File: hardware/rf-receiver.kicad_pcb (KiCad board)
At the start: 4 copper layers, 90.8 x 50 mm, 160 parts, among them CON1 FPC_6POS, IC1 ATSAMD21G18A-AU, IC2 AD9954, IC3 74LVC74, J1 Conn_01x05_Female, J2 Conn_Coaxial, J3 USB_C_Receptacle, P1 ROT_ENC, SW1 BTN1, SW2 BTN2, SW3 BTN3, U1 74HC14, U10 TPS62173DSG, U11 MIC5504-1.8YM5, U12 MIC5504-1.8YM5, U2 RC1602A, U3 TXB0108PWR, U4 MIC5504-3.3YM5, U5 OPA300, U7 Transformer, U8 NE5532, U9 74CBTLV3253, Y1 Crystal_Small

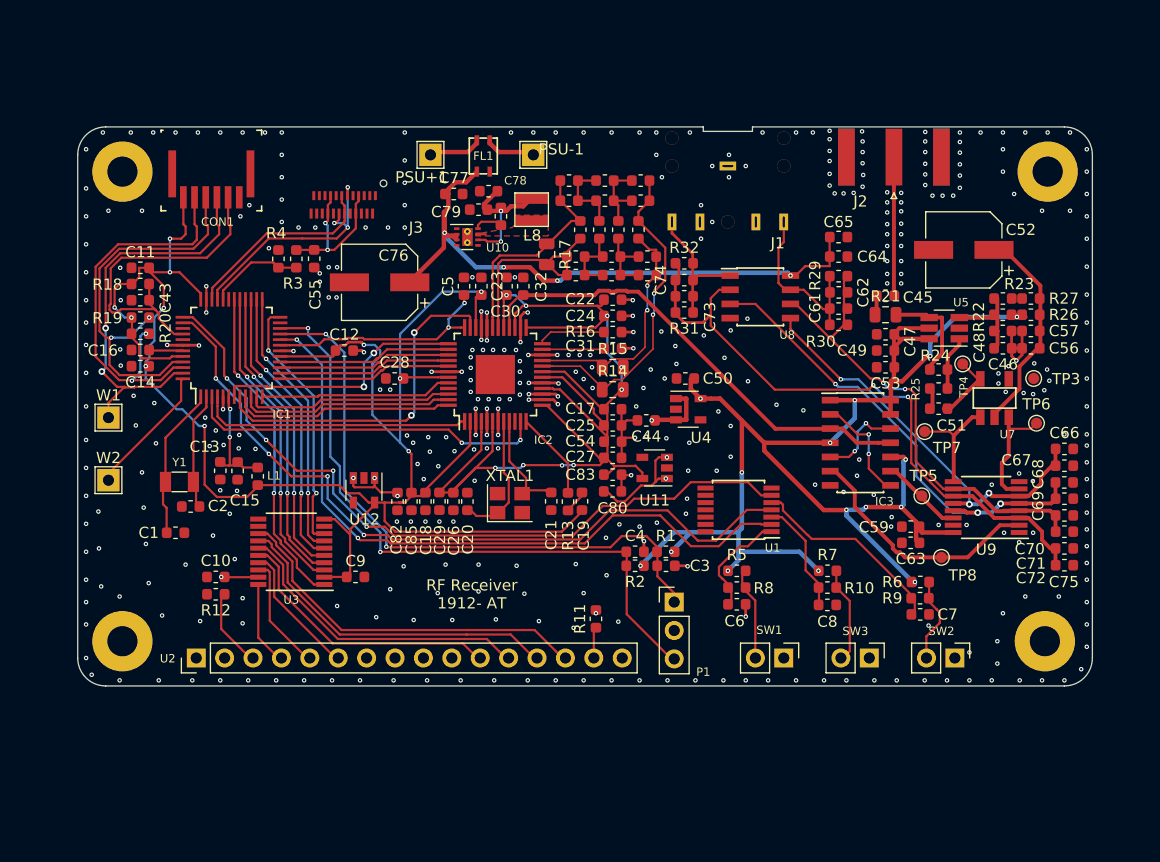
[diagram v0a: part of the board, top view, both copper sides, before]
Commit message: Added rpi changes - seems weird that I forgot that for so long
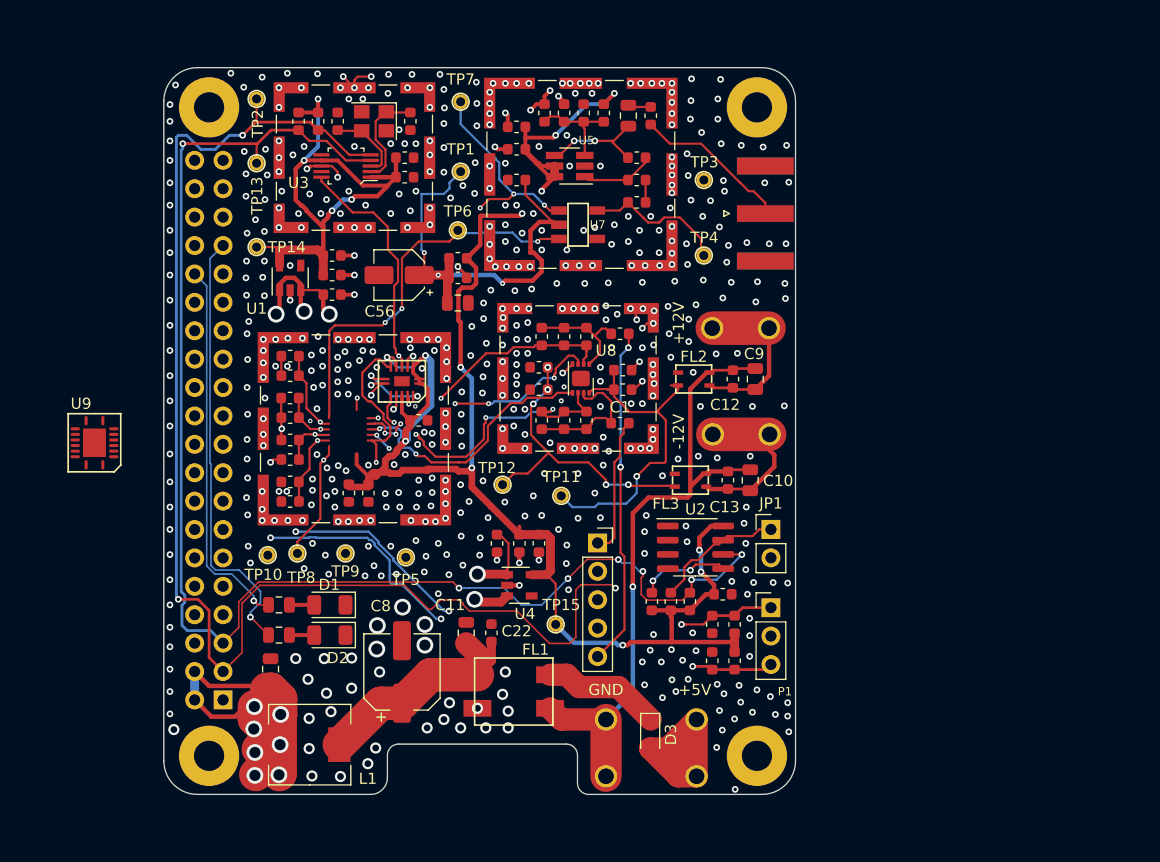
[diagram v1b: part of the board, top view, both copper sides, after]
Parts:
- removed C24, C25, C26, C27, C28, C29, C30, C43, C54, C77, C79, C80, C82: 100nF, Capacitor_SMD:C_0603_1608Metric
- removed C31: 1uF, Capacitor_SMD:C_0603_1608Metric
- removed C32, C33, C37, C38: 22pF, Capacitor_SMD:C_0603_1608Metric
- removed C34, C35, C39: 39pF, Capacitor_SMD:C_0603_1608Metric
- removed C36, C42: 33pF, Capacitor_SMD:C_0603_1608Metric
- removed C40, C41: 7.5pF, Capacitor_SMD:C_0603_1608Metric
- removed C55: C_Small, Capacitor_SMD:C_0603_1608Metric
- removed C76: 100uF, Capacitor_SMD:CP_Elec_6.3x7.7
- removed C78: 22uF, Capacitor_SMD:C_0603_1608Metric
- removed C83, C85: 10uF, Capacitor_SMD:C_0603_1608Metric
- removed CON1: FPC_6POS, FPC_conn:HFW6R_2STE1LF
- removed IC1: ATSAMD21G18A-AU, Package_QFP:TQFP-48_7x7mm_P0.5mm
- removed IC2: AD9954, Package_QFP:TQFP-48-1EP_7x7mm_P0.5mm_EP3.5x3.5mm
- removed L2, L3: 12nH, Inductor_SMD:L_0603_1608Metric
- removed L4, L5: 18nH, Inductor_SMD:L_0603_1608Metric
- removed L6, L7: 20nH, Inductor_SMD:L_0603_1608Metric
- removed L8: 2.2uH, athir:XFL3012
- removed PSU+1: PSU+, TestPoint:TestPoint_THTPad_2.0x2.0mm_Drill1.0mm
- removed PSU-1: PSU-, TestPoint:TestPoint_THTPad_2.0x2.0mm_Drill1.0mm
- removed R10, R30, R32: 10kohm, Resistor_SMD:R_0603_1608Metric
- removed R11: 220ohm, Resistor_SMD:R_0603_1608Metric
- removed R12: 2kohm, Resistor_SMD:R_0603_1608Metric
- removed R13: 243ohm, Resistor_SMD:R_0603_1608Metric
- removed R14, R15, R17: 50ohm, Resistor_SMD:R_0805_2012Metric
- removed R16: 3.92kohm, Resistor_SMD:R_0603_1608Metric
- removed R18, R19, R20: 100kohm, Resistor_SMD:R_0603_1608Metric
- removed R33: 100k, Resistor_SMD:R_0603_1608Metric
- removed SW1: BTN1, Connector_PinHeader_2.54mm:PinHeader_1x02_P2.54mm_Vertical
- removed SW2: BTN2, Connector_PinHeader_2.54mm:PinHeader_1x02_P2.54mm_Vertical
- removed SW3: BTN3, Connector_PinHeader_2.54mm:PinHeader_1x02_P2.54mm_Vertical
- removed U10: TPS62173DSG, Package_SON:WSON-8-1EP_2x2mm_P0.5mm_EP0.9x1.6mm_ThermalVias
- removed U11, U12: MIC5504-1.8YM5, Package_TO_SOT_SMD:SOT-23-5
- removed W1: TX, TestPoint:TestPoint_THTPad_2.0x2.0mm_Drill1.0mm
- removed W2: RX, TestPoint:TestPoint_THTPad_2.0x2.0mm_Drill1.0mm
- removed XTAL1: 25MHz 20pF, Crystal:Crystal_SMD_3225-4Pin_3.2x2.5mm
- added D1: LED, Diode_SMD:D_1206_3216Metric, F.Cu at (89.8, 105.8)
- added D2: LED, Diode_SMD:D_1206_3216Metric, F.Cu at (89.8, 108.5)
- added D3: D_Small_ALT, Diode_SMD:D_SOD-323_HandSoldering, F.Cu at (118.5, 117.3)
- added FL2: ACP3225, athir:ACP3225, F.Cu at (122.3, 85.5)
- added FL3: ACP3225, athir:ACP3225, F.Cu at (122.0, 94.6)
- added J10: 12P_VIN, athir:FASTON63951-1, F.Cu at (124.0, 81.0)
- added J12: 12N_VIN, athir:FASTON63951-1, F.Cu at (124.0, 90.5)
- added J4: 5_VIN, athir:FASTON63951-1, F.Cu at (122.6, 116.0)
- added J5: RF_Shield_One_Piece, RF_Shielding:Laird_Technologies_BMI-S-102_16.50x16.50mm, F.Cu at (112.2, 67.2)
- added J6: RF_Shield_One_Piece, RF_Shielding:Laird_Technologies_BMI-S-101_13.66x12.70mm, F.Cu at (112.0, 85.5)
- added J7: RF_Shield_One_Piece, RF_Shielding:Laird_Technologies_BMI-S-102_16.50x16.50mm, F.Cu at (92.0, 90.0)
- added J8: RF_Shield_One_Piece, RF_Shielding:Laird_Technologies_BMI-S-101_13.66x12.70mm, F.Cu at (92.0, 65.8)
- added J9: GND_IN, athir:FASTON63951-1, F.Cu at (114.5, 116.0)
- added JP1: Jumper_2_Open, Connector_PinHeader_2.54mm:PinHeader_1x02_P2.54mm_Vertical, F.Cu at (129.2, 99.0)
- added REF**: RPIHAT, athir:RPIHAT, F.Cu at (103.2, 90.2)
- added TP1: RF_DC_BIAS, athir:testpoint_probe, F.Cu at (101.5, 67.0)
- added TP10: 5V_TP, athir:testpoint_probe, F.Cu at (84.2, 101.3)
- added TP11: 12V_TP, athir:testpoint_probe, F.Cu at (110.5, 96.0)
- added TP12: -12V_TP, athir:testpoint_probe, F.Cu at (105.2, 95.0)
- added TP13: SCL, athir:testpoint_probe, F.Cu at (83.2, 66.2)
- added TP14: 3.3VA, athir:testpoint_probe, F.Cu at (83.2, 73.8)
- added TP15: 3.3V, athir:testpoint_probe, F.Cu at (110.0, 107.5)
- added TP2: SDA, athir:testpoint_probe, F.Cu at (83.2, 60.5)
- added TP9: GND, athir:testpoint_probe, F.Cu at (91.2, 101.2)
- C1, C2: value 15pF -> DC BLOCK
- C10, C9: value 0.1uF -> 22uF; footprint Capacitor_SMD:C_0603_1608Metric -> Capacitor_SMD:C_0805_2012Metric
- C11: value 10uF -> 22uF; footprint Capacitor_SMD:C_0603_1608Metric -> Capacitor_SMD:C_0805_2012Metric
- C13: value 10uF -> 100nF
- C14, C15: value 100nF -> 39pF
- C18, C44, C5: value 100nF -> 10uF
- C19: value 10nF -> 10uF
- C20, C21: value 39pF -> 100nF
- C52: value 47uF -> 22uF; footprint Capacitor_SMD:CP_Elec_6.3x7.7 -> Capacitor_SMD:C_0805_2012Metric
- C56: footprint Capacitor_SMD:C_0603_1608Metric -> Capacitor_SMD:CP_Elec_4x5.4
- C6: value 100nF -> 10nF
- C7: value 100nF -> 22uF; footprint Capacitor_SMD:C_0603_1608Metric -> Capacitor_SMD:C_0805_2012Metric
- C8: value 100nF -> 47uF/100uF; footprint Capacitor_SMD:C_0603_1608Metric -> Capacitor_SMD:CP_Elec_6.3x5.4
- FL1: value ACP3225 -> ACM90V-701-2PL-TL00; footprint athir:ACP3225 -> athir:ACM70V-701-2PL-TL00
- IC3: value 74LVC74 -> 74LVC74ABQ; footprint Package_SO:SOIC-14_3.9x8.7mm_P1.27mm -> athir:DHVQFN14
- J1: value Conn_01x05_Female -> InputConP6; footprint athir:SJ1-35235 -> Connector_PinSocket_2.54mm:PinSocket_1x05_P2.54mm_Vertical
- J3: value USB_C_Receptacle -> Raspberry_Pi_2_3; footprint athir:DX07S024JJ -> Connector_PinSocket_2.54mm:PinSocket_2x20_P2.54mm_Vertical; moved to B.Cu
- L1: value SMD-FERRITE-CHIP-120-OHM-500MA_0603_ -> 47+uH; footprint Capacitor_SMD:C_0603_1608Metric -> Inductor_SMD:L_Wuerth_HCM-7050
- R3: value R_Small -> 100; footprint Resistor_SMD:R_0603_1608Metric -> Resistor_SMD:R_0805_2012Metric
- R4: value R_Small -> 1k
- R5, R8: value 10kohm -> 3k9
- R6, R7: value 10kohm -> I2CPULLUP
- R9: value 10kohm -> 100; footprint Resistor_SMD:R_0603_1608Metric -> Resistor_SMD:R_0805_2012Metric
- TP3, TP4, TP5, TP6, TP7, TP8: footprint TestPoint:TestPoint_Pad_D1.0mm -> athir:testpoint_probe
- U1: value 74HC14 -> MIC5504-3.3YM5; footprint Package_SO:TSSOP-14_4.4x5mm_P0.65mm -> Package_TO_SOT_SMD:SOT-23-5
- U2: value RC1602A -> CAT24C128; footprint Connector_PinHeader_2.54mm:PinHeader_1x16_P2.54mm_Vertical -> Package_SO:SOIC-8_3.9x4.9mm_P1.27mm
- U3: value TXB0108PWR -> SI5351A-B-GT; footprint Package_SO:TSSOP-20_4.4x6.5mm_P0.65mm -> digikey-footprints:MSOP-10_W3mm
- U8: value NE5532 -> OPA167B-DRG; footprint Package_SO:SOIC-8_3.9x4.9mm_P1.27mm -> Package_SON:SON-8-1EP_3x2mm_P0.5mm_EP1.4x1.6mm
- U9: footprint Package_SO:TSSOP-16_4.4x5mm_P0.65mm -> athir:PVQFN16
- Y1: value Crystal_Small -> 25MHz 20pF; footprint Crystal:Crystal_SMD_3215-2Pin_3.2x1.5mm -> Crystal:Crystal_SMD_3225-4Pin_3.2x2.5mm
- moved U9 80.0 mm to (68.8, 91.2)
- moved C66 69.7 mm to (86.2, 83.5), turned to 180 degrees
- moved C67 69.7 mm to (86.2, 85.2), turned to 180 degrees
- moved C68 69.7 mm to (86.2, 87.2), turned to 180 degrees
- moved C69 69.6 mm to (86.2, 89.0), turned to 180 degrees
- moved C70 69.6 mm to (86.2, 91.0), turned to 180 degrees
- moved C71 69.5 mm to (86.2, 92.8), turned to 180 degrees
- moved C72 69.5 mm to (86.2, 94.8), turned to 180 degrees
- moved C75 69.5 mm to (86.2, 96.5), turned to 180 degrees
- moved R6 69.2 mm to (87.0, 62.5), turned to 270 degrees
- moved R7 60.8 mm to (88.8, 62.5), turned to 270 degrees
- moved C7 58.3 mm to (84.5, 111.5), turned to 90 degrees
- moved TP8 57.6 mm to (86.9, 101.2), turned to 180 degrees
- moved R9 57.4 mm to (85.2, 108.5), turned to 0 degrees
- moved C56 56.9 mm to (96.0, 76.2)
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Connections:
- C1 pad 1: Net-(C1-Pad1) -> /I_OUT
- C1 pad 2: GND -> /right
- C10 pad 1: +5V -> Net-(C10-Pad1)
- C10 pad 2: GND -> Net-(C10-Pad2)
- C11 pad 1: +1V8 -> Net-(C11-Pad1)
- C12 pad 1: +1V8 -> Net-(C12-Pad1)
- C12 pad 2: GND -> Net-(C10-Pad2)
- C13 pad 1: /VDDANA -> Net-(C10-Pad1)
- C13 pad 2: GND -> Net-(C10-Pad2)
- C14 pad 1: +1V8 -> GND
- C14 pad 2: GND -> Net-(C14-Pad2)
- C15 pad 1: /VDDANA -> GND
- C15 pad 2: GND -> Net-(C15-Pad2)
- C16 pad 1: /VDDCORE -> +3.3VA
- C17 pad 2: VAA -> +3.3VA
- C18 pad 1: GND -> +5V
- C18 pad 2: +1V8 -> GND
- C19 pad 1: Net-(C19-Pad1) -> +3.3VA
- C19 pad 2: +1V8 -> GND
- C2 pad 1: Net-(C2-Pad1) -> /Q_OUT
- C2 pad 2: GND -> /left
- C20 pad 1: GND -> +3.3VA
- C20 pad 2: Net-(C20-Pad2) -> GND
- C21 pad 1: Net-(C21-Pad1) -> +3V3
- C22 pad 1: GND -> Net-(C11-Pad1)
- C22 pad 2: VAA -> GND
- C23 pad 2: +1V8 -> +3V3
- C5 pad 1: /DDS_RESET -> GND
- C5 pad 2: GND -> -12V
- C6 pad 1: Net-(C6-Pad1) -> GND
- C6 pad 2: GND -> -12V
- C61 pad 1: /Tayoe Mixer sheet/I_OUT -> /I_OUT
- C62 pad 1: /Tayoe Mixer sheet/I_OUT -> /I_OUT
- C7 pad 1: Net-(C7-Pad1) -> +5V
- C73 pad 1: /Tayoe Mixer sheet/Q_OUT -> /Q_OUT
- C74 pad 1: /Tayoe Mixer sheet/Q_OUT -> /Q_OUT
- C8 pad 1: Net-(C8-Pad1) -> Net-(C11-Pad1)
- C9 pad 1: +1V8 -> Net-(C12-Pad1)
- C9 pad 2: GND -> Net-(C10-Pad2)
- FL1 pad 1: +12V -> Net-(C10-Pad2)
- FL1 pad 2: GND -> Net-(D3-Pad1)
- FL1 pad 3: Net-(FL1-Pad3) -> Net-(C11-Pad1)
- FL1 pad 4: Net-(FL1-Pad4) -> GND
- IC3 pad 11: /AD9954sheet/COMP_OUT -> /Tayoe Mixer sheet/LO_IN
- IC3 pad 3: /AD9954sheet/COMP_OUT -> /Tayoe Mixer sheet/LO_IN
- J1 pad 1: GND -> /right
- J1 pad 2: /Tayoe Mixer sheet/Q_OUT -> (no net)
- J1 pad 3: /Tayoe Mixer sheet/I_OUT -> GND
- J1 pad 4: GND -> (no net)
- J1 pad 5: Net-(J1-Pad5) -> /left
- L1 pad 1: +1V8 -> Net-(C11-Pad1)
- L1 pad 2: /VDDANA -> +5V
- R29 pad 1: /Tayoe Mixer sheet/I_OUT -> /I_OUT
- R3 pad 1: /USB_VCC -> Net-(J3-Pad32)
- R3 pad 2: Net-(C55-Pad1) -> Net-(D1-Pad2)
- R31 pad 1: /Tayoe Mixer sheet/Q_OUT -> /Q_OUT
- R4 pad 1: /USB_VCC -> +3V3
- R4 pad 2: GND -> Net-(JP1-Pad1)
- R5 pad 2: Net-(R5-Pad2) -> /SCL
- R6 pad 1: +3V3 -> +3.3VA
- R6 pad 2: Net-(R6-Pad2) -> /SCL
- R7 pad 1: +3V3 -> +3.3VA
- R7 pad 2: Net-(R10-Pad1) -> /SDA
- R8 pad 1: Net-(R5-Pad2) -> +3V3
- R8 pad 2: Net-(C6-Pad1) -> /SDA
- R9 pad 1: Net-(R6-Pad2) -> Net-(J3-Pad33)
- R9 pad 2: Net-(C7-Pad1) -> Net-(D2-Pad2)
- U1 pad 1: Net-(C6-Pad1) -> +5V
- U1 pad 2: /BTN1 -> GND
- U1 pad 3: Net-(C8-Pad1) -> +5V
- U1 pad 4: /BTN3 -> (no net)
- U1 pad 5: Net-(C7-Pad1) -> +3.3VA
- U2 pad 2: +5V -> GND
- U2 pad 3: Net-(R12-Pad1) -> GND
- U2 pad 4: Net-(U2-Pad4) -> GND
- U2 pad 5: Net-(U2-Pad5) -> /SDA
- U2 pad 6: Net-(U2-Pad6) -> /SCL
- U2 pad 7: Net-(U2-Pad7) -> Net-(JP1-Pad1)
- U2 pad 8: Net-(U2-Pad8) -> +3V3
- U3 pad 1: /LCD_RS -> +3.3VA
- U3 pad 10: +1V8 -> /Tayoe Mixer sheet/LO_IN
- U3 pad 2: +1V8 -> Net-(C15-Pad2)
- U3 pad 3: /LCD_RW -> Net-(C14-Pad2)
- U3 pad 4: /LCD_EN -> /SCL
- U3 pad 5: /LCD_D4 -> /SDA
- U3 pad 6: /LCD_D5 -> (no net)
- U3 pad 7: /LCD_D6 -> +3.3VA
- U3 pad 8: /LCD_D7 -> GND
- U3 pad 9: Net-(U3-Pad9) -> (no net)
- U4 pad 4: Net-(U4-Pad4) -> (no net)
- U8 pad 1: /Tayoe Mixer sheet/Q_OUT -> /Q_OUT
- U8 pad 4: GND -> -12V
- U8 pad 7: /Tayoe Mixer sheet/I_OUT -> /I_OUT
- Y1 pad 1: Net-(C1-Pad1) -> Net-(C15-Pad2)
- Y1 pad 2: Net-(C2-Pad1) -> GND
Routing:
- net +1V8: track 168.2 -> 0.00 mm, vias 11 -> 0
- net /SDA: track 0.00 -> 133.2 mm, vias 0 -> 5
- net /SCL: track 0.00 -> 127.4 mm, vias 0 -> 7
- net VAA: track 107.1 -> 0.00 mm, vias 9 -> 0
- net /BTN3: track 68.0 -> 0.00 mm, vias 4 -> 0
- net /BTN2: track 67.0 -> 0.00 mm, vias 4 -> 0
- net /BTN1: track 61.7 -> 0.00 mm, vias 2 -> 0
- net Net-(C10-Pad2): track 0.00 -> 58.3 mm, vias 0 -> 1
- net +3.3VA: track 0.00 -> 52.2 mm, vias 0 -> 4
- net /AD9954sheet/COMP_OUT: track 42.4 -> 0.00 mm
- net Net-(J3-Pad33): track 0.00 -> 39.5 mm, vias 0 -> 1
- net /JTAGConn58895F8D/SWDIO: track 36.0 -> 0.00 mm, vias 2 -> 0
- net /UART_TX: track 35.9 -> 0.00 mm, vias 2 -> 0
- net /JTAGConn58895F8D/SWCLK: track 35.3 -> 0.00 mm, vias 2 -> 0
- net Net-(J3-Pad32): track 0.00 -> 33.8 mm, vias 0 -> 1
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- removed copper zone on F.Cu, net Net-(L8-Pad1)
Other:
- board size 90.8 x 50 mm -> 56.5 x 65 mm
- net class PWR: via_dia 0.6 -> 1.5; via_drill 0.4 -> 1
- net class PWR_1 added: clearance 0.15, trace_width 0.3, via_dia 0.6, via_drill 0.3
- net class RF added: clearance 0.15, trace_width 0.2, via_dia 0.45, via_drill 0.2
- board text added: "+12V"
- board text added: "+5V"
- board text added: "-12V"
- board text added: "AUDIO AMPS"
- board text added: "BUFFER 1:4 BALUN"
- board text added: "CLOCK"
- board text added: "Detector"
- board text added: "GND"
- board text added: "RF SHIELD 1950 - AT"
- board text removed: "RF Receiver 1912- AT"
